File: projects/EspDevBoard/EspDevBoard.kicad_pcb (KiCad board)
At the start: 2 copper layers, 0 parts

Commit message: start with pcb
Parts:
- added C1: 4u7F, frep:C0805, F.Cu at (177.8, 81.3)
- added C10: 100nF, frep:C0805, B.Cu at (146.1, 117.3)
- added C11: 1uF, frep:C0805, B.Cu at (131.3, 122.9)
- added C12: 100nF, frep:C0805, F.Cu at (165.9, 110.5)
- added C13: 100nF, frep:C0805, F.Cu at (165.6, 92.7)
- added C2: 4u7F, frep:C0805, F.Cu at (115.6, 108.0)
- added C3: 100nF, frep:C0805, B.Cu at (167.6, 81.3)
- added C4: 4u7F, frep:C0805, B.Cu at (165.1, 81.3)
- added C5: 10uF, frep:C0805, F.Cu at (174.2, 100.1)
- added C6: 100nF, frep:C0805, B.Cu at (139.7, 121.9)
- added C7: 100nF, frep:C0805, F.Cu at (176.8, 100.1)
- added C8: 1uF, frep:C0805, F.Cu at (181.6, 96.8)
- added C9: 100nF, frep:C0805, B.Cu at (140.2, 118.9)
- added CON1: USB-MICRO, frep:USB_Micro, F.Cu at (114.3, 85.1)
- added D1: DIODE, frep:Diode-MiniMELF_Handsoldering, B.Cu at (150.9, 120.4)
- added D2: LED, frep:LED-0805, F.Cu at (137.9, 105.4)
- added F1: FUSE, frep:C1812, F.Cu at (121.9, 77.5)
- added JP1: JUMPER3, frep:Pin_Proto_Straight_1x03, F.Cu at (127.0, 90.2)
- added JP2: JUMPER3, frep:Pin_Proto_Straight_1x03, F.Cu at (123.2, 90.2)
- added L1: INDUCTOR, frep:C0805, B.Cu at (133.6, 122.9)
- added P1: ICSP, frep:Pin_Proto_Straight_2x03, F.Cu at (151.1, 129.5)
- added P2: ICSP_P, frep:Pin_Proto_Straight_2x03, F.Cu at (134.6, 129.5)
- added P3: Display, frep:Pin_Proto_Straight_2x10, B.Cu at (174.0, 129.5)
- added P4: Sepic_TH, frep:Sepic_TH, F.Cu at (174.0, 101.6)
- added R1: 33, frep:R0805, B.Cu at (170.2, 81.3)
- added R10: 10K, frep:R0805, F.Cu at (181.6, 118.1)
- added R11: 10R, frep:R0805, F.Cu at (169.7, 111.8)
- added R12: 10R, frep:R0805, F.Cu at (169.7, 109.2)
- added R13: 10R, frep:R0805, F.Cu at (168.9, 94.2)
- added R14: 10R, frep:R0805, F.Cu at (168.9, 91.4)
- added R15: 10K, frep:R0805, B.Cu at (136.4, 105.9)
- added R16: 330R, frep:R0805, B.Cu at (135.4, 102.6)
- added R17: 0.1R 1%, frep:R1206, F.Cu at (163.1, 110.5)
- added R18: 0.1R 1%, frep:R1206, F.Cu at (163.1, 92.7)
- added R19: 1K, frep:R0805, B.Cu at (134.6, 110.2)
- added R2: 33, frep:R0805, B.Cu at (172.7, 81.3)
- added R3: 10K, frep:R0805, B.Cu at (140.0, 85.9)
- added R4: 10K, frep:R0805, B.Cu at (150.9, 93.5)
- added R5: 10K, frep:R0805, B.Cu at (150.9, 98.0)
- added R6: 10K, frep:R0805, B.Cu at (150.9, 95.8)
- added R7: 10K, frep:R0805, B.Cu at (140.0, 89.9)
- added R8: 10K, frep:R0805, B.Cu at (139.7, 124.5)
- added R9: 10K, frep:R0805, F.Cu at (180.3, 114.3)
- added S1: Reset, frep:TACTILE-PTH, F.Cu at (113.5, 129.0)
- added S2: User button, frep:TACTILE-PTH, F.Cu at (102.4, 129.0)
- added U1: ESP-12E, frep:ESP-12E, F.Cu at (135.4, 85.9)
- added U2: NODE_MCU, frep:NodeMcu, F.Cu at (143.5, 101.6)
- added U3: AZ1117, frep:SOT223, F.Cu at (113.0, 99.1)
- added U4: AD5274, frep:MSOP10, F.Cu at (181.6, 100.1)
- added U5: ATMEGA32U4, frep:TQFP44, F.Cu at (142.2, 114.3)
- added U6: INA219_SOT23_8, frep:SOT-23-8, F.Cu at (175.0, 110.7)
- added U7: INA219_SOT23_8, frep:SOT-23-8, F.Cu at (174.0, 93.0)
- added X1: Resonator, frep:Resonator, B.Cu at (144.3, 114.3)
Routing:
- net 3V3: track 0.00 -> 44.6 mm
- net GND: track 0.00 -> 27.3 mm, vias 0 -> 1
- net MOSI: track 0.00 -> 25.4 mm, vias 0 -> 1
- net RS: track 0.00 -> 25.2 mm, vias 0 -> 1
- net SCLK: track 0.00 -> 23.0 mm, vias 0 -> 1
- net RES: track 0.00 -> 22.9 mm
- net En+: track 0.00 -> 20.6 mm, vias 0 -> 1
- net Vin-: track 0.00 -> 15.5 mm
- net BootMode: track 0.00 -> 9.48 mm, vias 0 -> 1
- net Vin+: track 0.00 -> 9.00 mm
- net CS: track 0.00 -> 8.96 mm, vias 0 -> 1
- net Vout+: track 0.00 -> 8.35 mm
- net Vout-: track 0.00 -> 8.24 mm
- net A_RX: track 0.00 -> 7.98 mm
- net A_TX: track 0.00 -> 7.26 mm
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
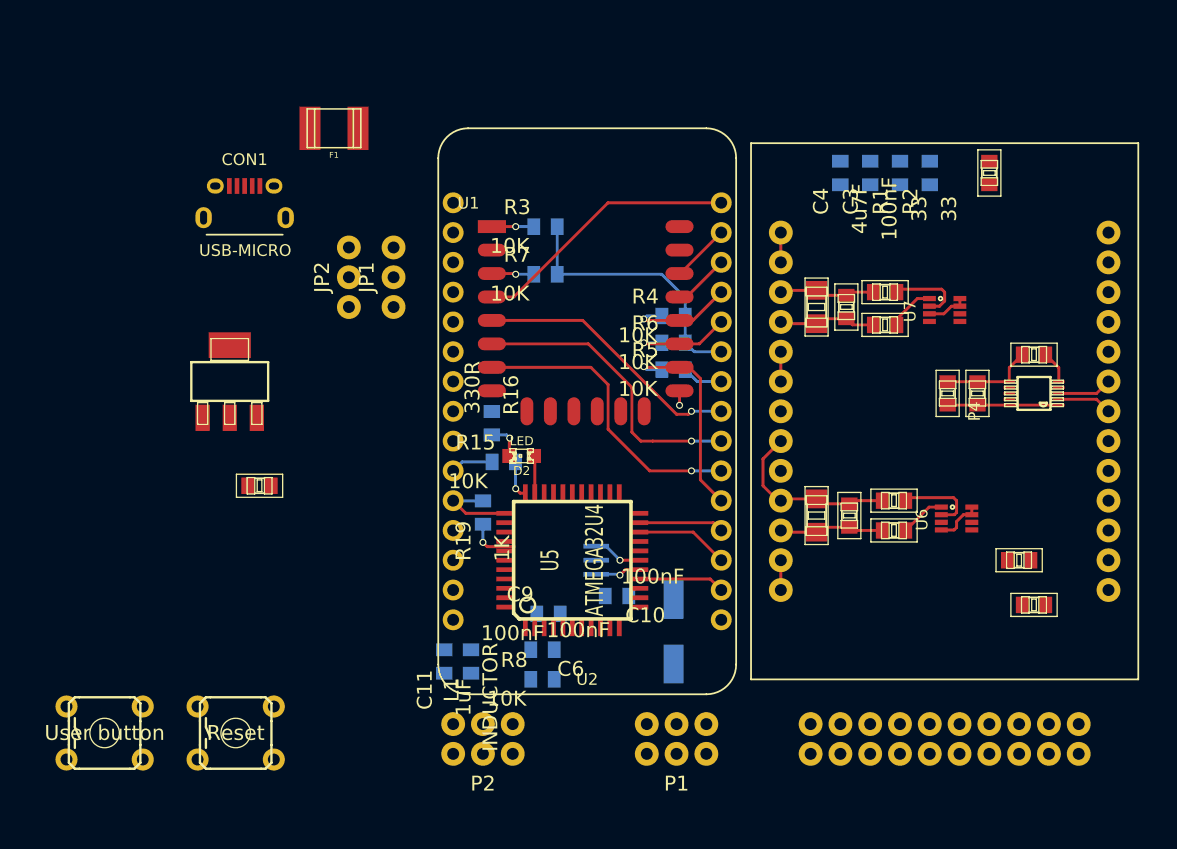
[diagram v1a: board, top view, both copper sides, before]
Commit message: work on espDevBoard
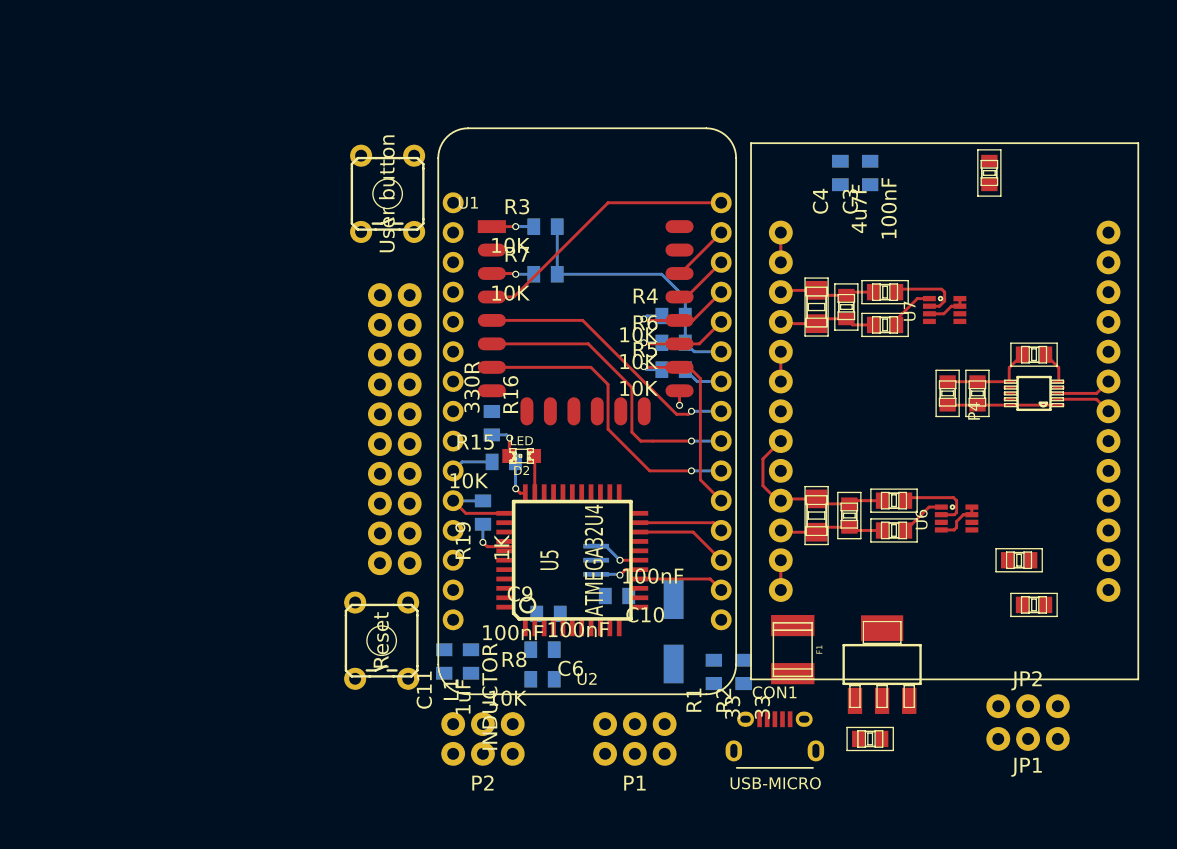
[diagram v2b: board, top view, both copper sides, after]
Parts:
- P3: footprint frep:Pin_Proto_Straight_2x10 -> frep:nhd-1.69-16028UGC3
- moved JP2 68.5 mm to (181.1, 126.7), turned to 0 degrees
- moved JP1 66.9 mm to (181.1, 129.5), turned to 180 degrees
- moved CON1 64.1 mm to (159.5, 130.6)
- moved U3 60.6 mm to (168.7, 123.2)
- moved F1 59.2 mm to (161.0, 121.9), turned to 270 degrees
- moved C2 56.4 mm to (167.6, 129.5)
- moved S2 51.9 mm to (126.5, 83.1), turned to 90 degrees
- moved R1 45.4 mm to (154.3, 123.8)
- moved R2 45.4 mm to (156.8, 123.8)
- moved P3 36.8 mm to (148.3, 103.1), turned to 270 degrees
- moved S1 14.7 mm to (126.0, 121.2), turned to 90 degrees
- moved P1 3.56 mm to (147.6, 129.5)

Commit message: work in progress
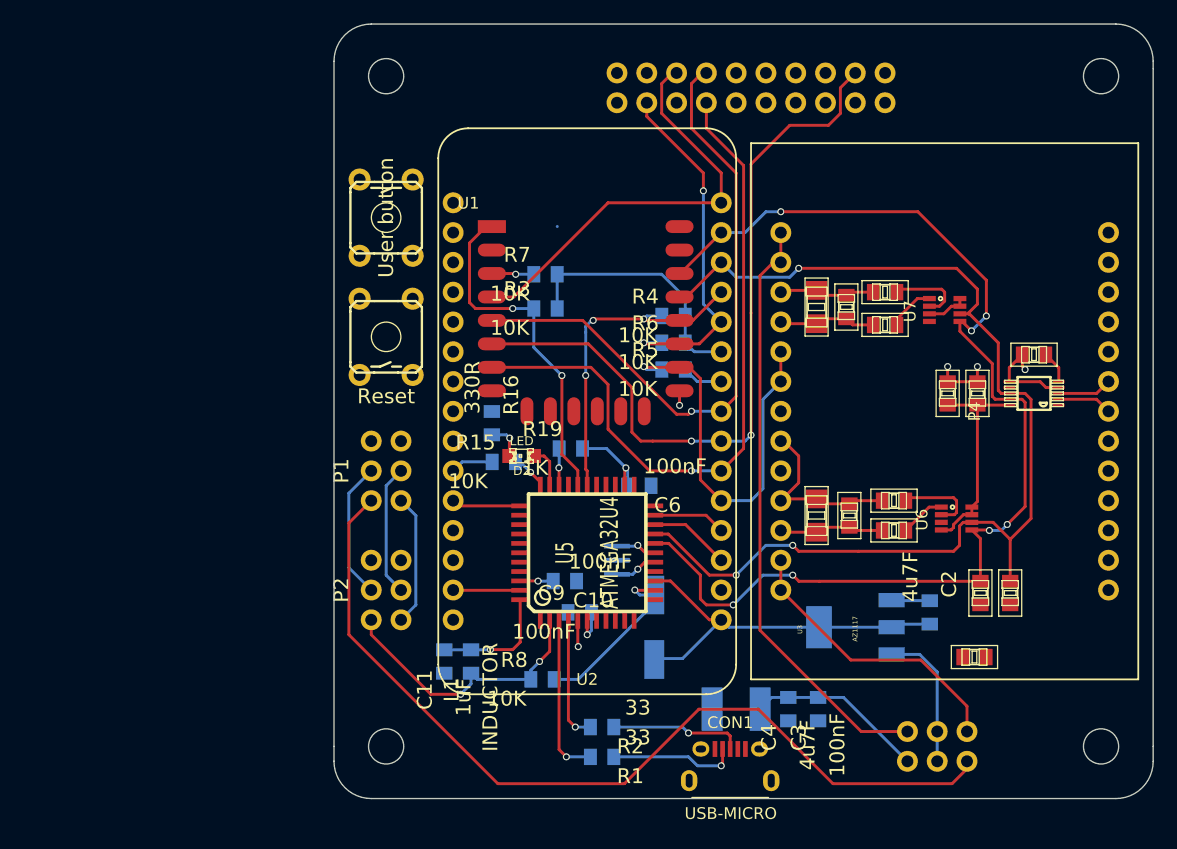
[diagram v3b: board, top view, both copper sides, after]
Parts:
- added P5: CONN_1, frep:MountingHole_3mm, F.Cu at (126.4, 130.2)
- added P6: CONN_1, frep:MountingHole_3mm, F.Cu at (187.3, 130.2)
- added P7: CONN_1, frep:MountingHole_3mm, F.Cu at (126.4, 73.0)
- added P8: CONN_1, frep:MountingHole_3mm, F.Cu at (187.3, 73.0)
- C2, F1, U3: moved to B.Cu
- moved C3 45.9 mm to (163.2, 127.0)
- moved C4 45.9 mm to (160.7, 127.0)
- moved C1 41.3 mm to (176.5, 122.6), turned to 0 degrees
- moved P1 31.2 mm to (126.4, 106.7), turned to 90 degrees
- moved S1 25.9 mm to (126.4, 95.2)
- moved C6 16.2 mm to (148.0, 108.0)
- moved P2 15.1 mm to (126.4, 116.8), turned to 90 degrees
- moved R2 12.9 mm to (144.8, 128.5), turned to 0 degrees
- moved P3 12.1 mm to (157.5, 95.2), turned to 180 degrees
- moved R1 12.0 mm to (144.8, 131.1), turned to 0 degrees
- moved C2 11.9 mm to (172.7, 118.7), turned to 90 degrees
- moved R19 9.27 mm to (142.1, 104.8), turned to 180 degrees
- moved JP2 9.06 mm to (173.4, 131.4), turned to 180 degrees
- moved JP1 7.77 mm to (173.4, 128.9)
- moved F1 7.01 mm to (156.2, 127.0), turned to 180 degrees
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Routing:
- net SCL: track 5.00 -> 98.9 mm, vias 0 -> 7
- net SDA: track 5.36 -> 94.6 mm, vias 0 -> 3
- net ICSP_Power: track 0.00 -> 76.6 mm
- net 3V3: track 44.6 -> 111.3 mm, vias 0 -> 3
- net Vout: track 2.54 -> 51.2 mm
- net RS: track 25.2 -> 64.5 mm, vias 1 -> 2
- net MOSI: track 25.4 -> 58.9 mm
- net SCLK: track 23.0 -> 54.7 mm
- net ESP_Reset: track 3.57 -> 29.9 mm, vias 1 -> 2
- net Vin: track 2.54 -> 24.7 mm
- net CS: track 8.96 -> 30.3 mm, vias 1 -> 2
- net BootMode: track 9.48 -> 28.3 mm, vias 1 -> 3
- net A_Reset: track 0.00 -> 15.4 mm, vias 0 -> 1
- net VBUS: track 0.00 -> 15.2 mm
- net D-: track 0.00 -> 14.0 mm, vias 0 -> 1
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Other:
- board outline added: 69.9 x 66 mm
